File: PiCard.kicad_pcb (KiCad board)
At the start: 4 copper layers, 81 x 50 mm, 54 parts, among them J1 Usb Data Jumper, J2 USB_C_Receptacle_USB2.0_16P, J3 UART Activity Jumper, J4 Bus_M.2_Socket_M, J5 Ethernet, J6 Micro_SD_Card_Det2, J7 nRPIBOOT Jumper, J8 RS232, M2_3V3 TestPoint, U1 TPD4EUSB30, U3 TPD4EUSB30, U4 TPD4EUSB30, U5 MAX3232, U6 RT9742GGJ5, U7 TPS82130

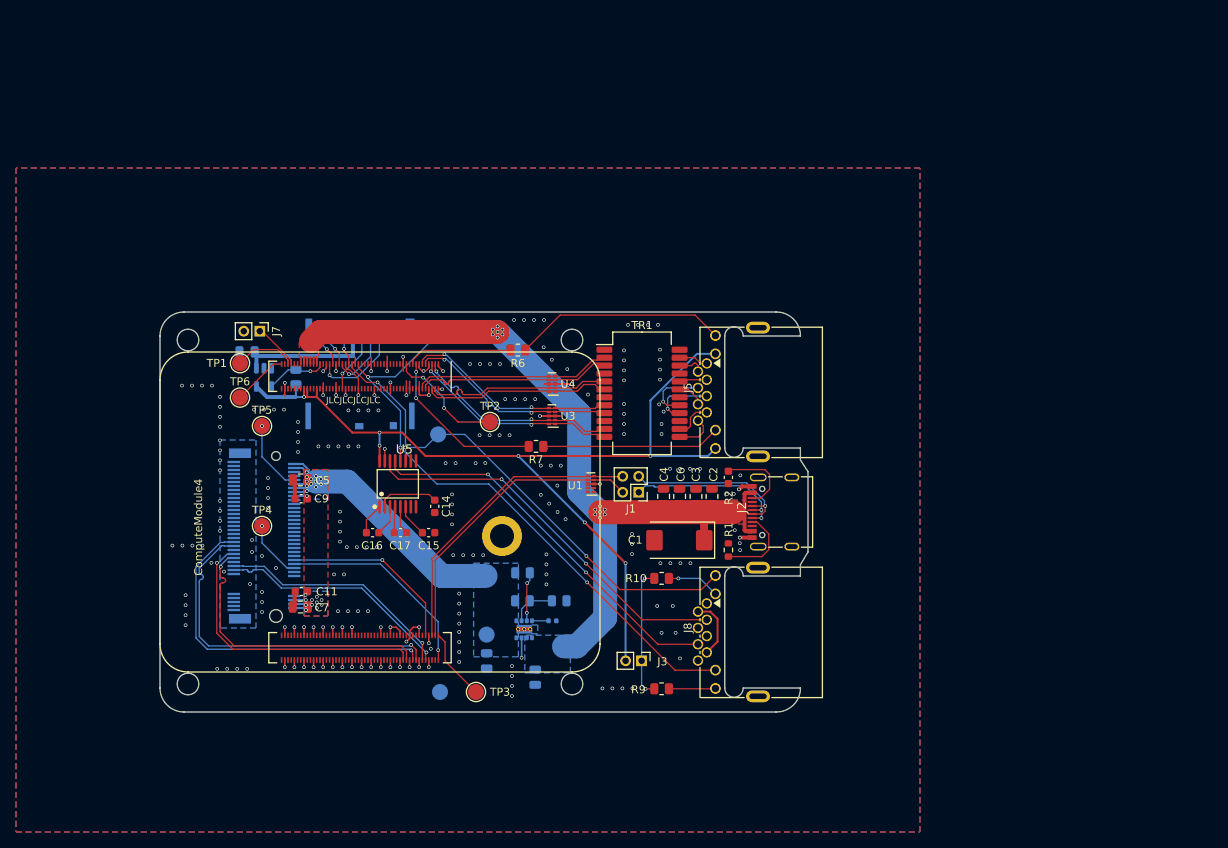
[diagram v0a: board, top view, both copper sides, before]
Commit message: update
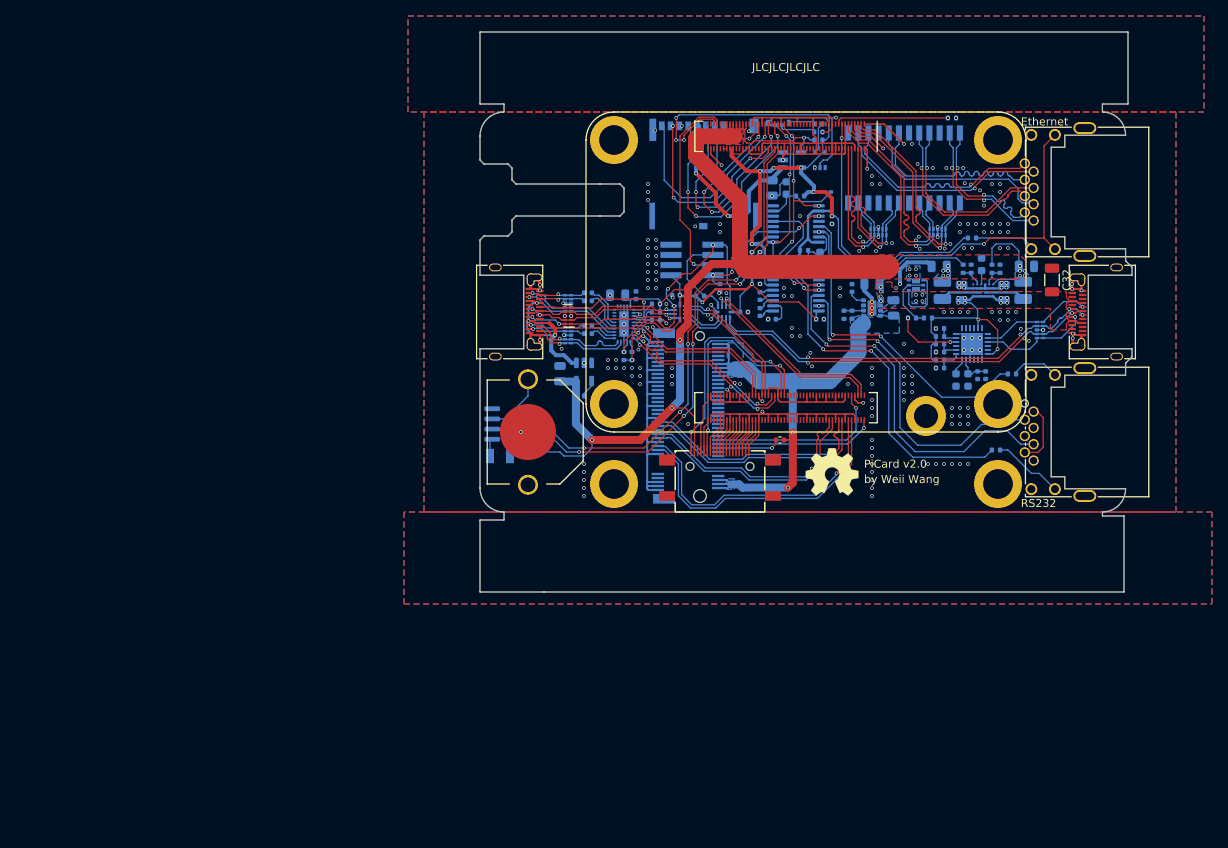
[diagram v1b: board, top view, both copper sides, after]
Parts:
- removed +5V1, GND1, GPIO14, GPIO15, M2_3V3, TP1, TP2, TP3, TP4, TP5, TP6: TestPoint, TestPoint:TestPoint_Pad_D2.0mm
- removed ComputeModule4: ComputeModule4-CM4, PiCard:Raspberry-Pi-4-Compute-Module
- removed J7: nRPIBOOT Jumper, Connector_PinHeader_2.00mm:PinHeader_1x02_P2.00mm_Vertical
- added BT1: RTC Battery, PiCard:BAT-SMD_MY-1220-03, F.Cu at (106.0, 90.0)
- added C13: 100n, Capacitor_SMD:C_0402_1005Metric, B.Cu at (163.2, 82.9)
- added C19: 22u, Capacitor_SMD:C_0805_2012Metric, B.Cu at (149.0, 71.5)
- added C20: 22u, Capacitor_SMD:C_0805_2012Metric, B.Cu at (151.7, 74.5)
- added C21: 430pF, Capacitor_SMD:C_0402_1005Metric, B.Cu at (146.5, 72.0)
- added C22: 100n, Capacitor_SMD:C_0402_1005Metric, B.Cu at (106.5, 92.5)
- added C23: 47u, Capacitor_SMD:C_0805_2012Metric, B.Cu at (110.0, 82.7)
- added C24: 47u, Capacitor_SMD:C_0805_2012Metric, B.Cu at (117.2, 72.9)
- added C25: 100n, Capacitor_SMD:C_0402_1005Metric, B.Cu at (119.5, 72.9)
- added C26: 100n, Capacitor_SMD:C_0402_1005Metric, B.Cu at (124.5, 72.9)
- added C27: 100n, Capacitor_SMD:C_0402_1005Metric, B.Cu at (113.5, 77.7)
- added C28: 100n, Capacitor_SMD:C_0402_1005Metric, B.Cu at (113.5, 76.7)
- added C29: 100n, Capacitor_SMD:C_0402_1005Metric, B.Cu at (133.0, 75.0)
- added C30: 100n, Capacitor_SMD:C_0402_1005Metric, B.Cu at (113.5, 72.6)
- added C31: 100n, Capacitor_SMD:C_0402_1005Metric, B.Cu at (113.5, 73.6)
- added C32: 2.2u, Capacitor_SMD:C_1206_3216Metric, F.Cu at (171.5, 71.0)
- added ComputeModule1: ComputeModule4-CM4, PiCard:Raspberry-Pi-4-Compute-Module, F.Cu at (116.8, 53.5)
- added D1: 1N5819WS, Diode_SMD:D_SOD-323, B.Cu at (140.0, 68.8)
- added D3: 1N5819WS, Diode_SMD:D_SOD-323, B.Cu at (142.8, 60.0)
- added D4: LED_Dual_AAKK, PiCard:LED-ARRAY-SMD_4P-L3.0-W1.5-L-FD, B.Cu at (137.3, 51.5)
- added H1: MountingHole, PiCard:MOUNTING-HOLE, F.Cu at (116.8, 96.5)
- added H2: MountingHole, PiCard:MOUNTING-HOLE, F.Cu at (164.8, 96.5)
- added L1: 1u, Inductor_SMD:L_1008_2520Metric, B.Cu at (167.9, 72.3)
- added L2: 1u, Inductor_SMD:L_1008_2520Metric, B.Cu at (157.8, 72.3)
- added Q1: DMP2065UFDB, PiCard:DFN200X200X60-8N, B.Cu at (154.5, 71.6)
- added R11: 680k 1%, Resistor_SMD:R_0402_1005Metric, B.Cu at (160.4, 69.6)
- added R12: 100k 1%, Resistor_SMD:R_0402_1005Metric, B.Cu at (161.4, 69.6)
- added R13: 5.1k, Resistor_SMD:R_0402_1005Metric, B.Cu at (157.5, 79.0)
- added R14: 1k, Resistor_SMD:R_0402_1005Metric, B.Cu at (157.5, 80.0)
- added R15: 150k 1%, Resistor_SMD:R_0402_1005Metric, B.Cu at (165.0, 69.6)
- added R17: 5.1k, Resistor_SMD:R_0402_1005Metric, B.Cu at (157.5, 81.0)
- added R18: 1k, Resistor_SMD:R_0402_1005Metric, B.Cu at (157.5, 82.0)
- added R19: 5.1k, Resistor_SMD:R_0402_1005Metric, B.Cu at (157.5, 78.1)
- added R20: 2.4k, Resistor_SMD:R_0402_1005Metric, B.Cu at (157.5, 77.1)
- added R22: 309k, Resistor_SMD:R_0402_1005Metric, B.Cu at (146.5, 75.3)
- added R23: 49.9k, Resistor_SMD:R_0402_1005Metric, B.Cu at (156.0, 75.7)
- added R24: 100k 1%, Resistor_SMD:R_0402_1005Metric, B.Cu at (145.5, 75.3)
- added R25: 1k, Resistor_SMD:R_0402_1005Metric, B.Cu at (154.0, 75.7)
- added R26: 5.1k, Resistor_SMD:R_0402_1005Metric, B.Cu at (135.0, 67.0)
- added R27: 5.1k, Resistor_SMD:R_0402_1005Metric, B.Cu at (134.0, 67.0)
- added R28: 12k, Resistor_SMD:R_0402_1005Metric, B.Cu at (112.5, 85.5)
- added R29: 909k, Resistor_SMD:R_0402_1005Metric, B.Cu at (122.0, 76.0)
- added R30: 12k, Resistor_SMD:R_0402_1005Metric, B.Cu at (127.5, 73.0)
- added R31: 200k, Resistor_SMD:R_0402_1005Metric, B.Cu at (119.0, 80.5)
- added R32: 200k, Resistor_SMD:R_0402_1005Metric, B.Cu at (122.0, 75.0)
- added R33: 499k, Resistor_SMD:R_0402_1005Metric, B.Cu at (122.0, 74.0)
- added R34: 12k, Resistor_SMD:R_0402_1005Metric, B.Cu at (118.0, 80.5)
- added R35: 12k, Resistor_SMD:R_0402_1005Metric, B.Cu at (130.0, 72.0)
- added R36: 1k, Resistor_SMD:R_0402_1005Metric, B.Cu at (142.3, 51.5)
- added SW1: SW_DIP_x04, PiCard:SW-SMD_8P-P1.27_EU-04KS, B.Cu at (126.5, 68.5)
- added SYM1: PiCard v2.0, PiCard:PICARD_NAMEPLATE, F.Cu at (144.0, 95.0)
- added U10: TPS2069C, Package_TO_SOT_SMD:SOT-23-5, B.Cu at (113.0, 82.5)
- added U11: TPD4EUSB30, Package_SON:USON-10_2.5x1.0mm_P0.5mm, B.Cu at (170.0, 77.2)
- added U12: TPD4EUSB30, Package_SON:USON-10_2.5x1.0mm_P0.5mm, F.Cu at (111.0, 75.5)
- added U13: TPD4EUSB30, Package_SON:USON-10_2.5x1.0mm_P0.5mm, B.Cu at (111.0, 77.9)
- added U14: TPD4EUSB30, Package_SON:USON-10_2.5x1.0mm_P0.5mm, B.Cu at (111.0, 73.9)
- added U15: TS3USB221, PiCard:RSE10, B.Cu at (130.5, 75.0)
- added U16: HD3SS3220, PiCard:RNH0030A, B.Cu at (118.0, 76.5)
- added U17: TS3USB221, PiCard:RSE10, B.Cu at (125.0, 75.0)
- added U18: 74LVC1G07, Package_TO_SOT_SMD:SOT-353_SC-70-5, B.Cu at (142.5, 56.0)
- added U2: SN74AHC123A, Package_SO:TSSOP-16_4.4x5mm_P0.65mm, B.Cu at (139.5, 64.0)
- added U8: TPS82130, PiCard:Texas_SIL0008D_MicroSiP-8-1EP_2.8x3mm_P0.65mm_EP1.1x1.9mm_ThermalVias, B.Cu at (149.0, 74.5)
- added U9: DS1307Z+, Package_SO:SOIC-8_3.9x4.9mm_P1.27mm, B.Cu at (104.0, 89.0)
- added Y1: 32.768kHz, Crystal:Crystal_SMD_3215-2Pin_3.2x1.5mm, B.Cu at (102.5, 93.0)
- C1: value 100uF -> 100n; footprint Capacitor_Tantalum_SMD:CP_EIA-7343-31_Kemet-D -> Capacitor_SMD:C_0402_1005Metric; moved to B.Cu
- C10: value 430pF -> 1u; footprint Capacitor_SMD:C_0402_1005Metric -> Capacitor_SMD:C_0603_1608Metric
- C11: value 100nF -> 1u; moved to B.Cu
- C12: value 22uF -> 100n; footprint Capacitor_SMD:C_0805_2012Metric -> Capacitor_SMD:C_0402_1005Metric
- C14, C15: value 100nF -> 22u; footprint Capacitor_SMD:C_0603_1608Metric -> Capacitor_SMD:C_0805_2012Metric; moved to B.Cu
- C16, C17: value 100nF -> 47u; footprint Capacitor_SMD:C_0603_1608Metric -> Capacitor_SMD:C_0805_2012Metric; moved to B.Cu
- C18: value 10uF -> 22n; footprint Capacitor_SMD:C_0805_2012Metric -> Capacitor_SMD:C_0603_1608Metric
- C2, C3, C4, C5, C7: value 10u -> 100n; footprint Capacitor_SMD:C_0805_2012Metric -> Capacitor_SMD:C_0402_1005Metric; moved to B.Cu
- C6: value 10u -> 1u; footprint Capacitor_SMD:C_0805_2012Metric -> Capacitor_SMD:C_0603_1608Metric; moved to B.Cu
- C8: value 22uF -> 1u; footprint Capacitor_SMD:C_0805_2012Metric -> Capacitor_SMD:C_0603_1608Metric
- C9: value 100nF -> 10u; footprint Capacitor_SMD:C_0603_1608Metric -> Capacitor_SMD:C_0805_2012Metric; moved to B.Cu
- J1: value Usb Data Jumper -> RS232; footprint Connector_PinHeader_2.00mm:PinHeader_2x02_P2.00mm_Vertical -> PiCard:RJ45-TH_RJ45-005-202-11
- J2: value USB_C_Receptacle_USB2.0_16P -> Ethernet; footprint PiCard:USB-C-SMD_TYPEC-304J-BCP16 -> PiCard:RJ45-TH_RJ45-005-202-11
- J3: value UART Activity Jumper -> Micro_SD_Card_Det2; footprint Connector_PinHeader_2.00mm:PinHeader_1x02_P2.00mm_Vertical -> PiCard:TF-SMD_503398-1892; moved to B.Cu
- J5: value Ethernet -> USB_C_Receptacle; footprint PiCard:RJ45-TH_MJ88B-B011-RVL11-P -> PiCard:USB-C-SMD_TYPE-C-31-M-27
- J6: value Micro_SD_Card_Det2 -> USB_C_Receptacle; footprint PiCard:TF-SMD_503398-1892 -> PiCard:USB-C-SMD_TYPE-C-31-M-27; moved to F.Cu
- J8: value RS232 -> HDMI_C_1.4; footprint PiCard:RJ45-TH_MJ88B-B011-RVL11-P -> PiCard:HDMI-SMD_19P-P0.40-H-F_HDMI-519S
- R1: value 5.1K -> 470; footprint Resistor_SMD:R_0603_1608Metric -> Resistor_SMD:R_0402_1005Metric; moved to B.Cu
- R10: value 470R -> 787k; footprint Resistor_SMD:R_0805_2012Metric -> Resistor_SMD:R_0402_1005Metric; moved to B.Cu
- R2: value 5.1K -> 470; footprint Capacitor_SMD:C_0603_1608Metric -> Resistor_SMD:R_0402_1005Metric; moved to B.Cu
- R3: value 100k -> 1k; footprint Resistor_SMD:R_0805_2012Metric -> Resistor_SMD:R_0402_1005Metric
- R4: value 309k -> 100k 1%; footprint Resistor_SMD:R_0805_2012Metric -> Resistor_SMD:R_0402_1005Metric
- R5: value 100k -> 100k 1%; footprint Resistor_SMD:R_0805_2012Metric -> Resistor_SMD:R_0402_1005Metric
- R6, R7: value 470R -> 470; footprint Resistor_SMD:R_0805_2012Metric -> Resistor_SMD:R_0402_1005Metric; moved to B.Cu
- R8: value 12K 1% -> 12k; footprint Resistor_SMD:R_0805_2012Metric -> Resistor_SMD:R_0402_1005Metric
- R9: value 470R -> 12k; footprint Resistor_SMD:R_0805_2012Metric -> Resistor_SMD:R_0402_1005Metric
- TR1: value 30F-51NL -> H2456G; footprint Transformer_SMD:Transformer_Ethernet_YDS_30F-51NL_SO-24_7.1x15.1mm -> PiCard:XFMR-SMD-24_L16.6-W9.0-LS9.6-BL; moved to B.Cu
- U1: value TPD4EUSB30 -> MAX3232; footprint Package_SON:USON-10_2.5x1.0mm_P0.5mm -> Package_SO:TSSOP-16_4.4x5mm_P0.65mm; moved to B.Cu
- U3, U4: moved to B.Cu
- U5: value MAX3232 -> RT9742GGJ5; footprint PiCard:TSSOP-16_L5.0-W4.4-P0.65-LS6.4-BL -> Package_TO_SOT_SMD:TSOT-23-5; moved to B.Cu
- U6: value RT9742GGJ5 -> TPS62180; footprint Package_TO_SOT_SMD:TSOT-23-5 -> PiCard:YZF0024AMAM
- U7: value TPS82130 -> CYPD3177-24LQ; footprint PiCard:Texas_SIL0008D_MicroSiP-8-1EP_2.8x3mm_P0.65mm_EP1.1x1.9mm_ThermalVias -> Package_DFN_QFN:QFN-24-1EP_4x4mm_P0.5mm_EP2.75x2.75mm
- moved C18 92.5 mm to (162.7, 69.0), turned to 90 degrees
- moved J6 92.1 mm to (176.8, 75.0), turned to 90 degrees
- moved U6 90.6 mm to (162.9, 72.3), turned to 90 degrees
- moved C16 88.2 mm to (168.3, 69.3)
- moved C11 87.4 mm to (161.0, 83.5), turned to 90 degrees
- moved C7 82.2 mm to (144.0, 63.5), turned to 90 degrees
- moved C14 76.0 mm to (165.5, 72.5), turned to 90 degrees
- moved C17 75.1 mm to (157.4, 69.3), turned to 180 degrees
- moved C15 73.1 mm to (160.2, 72.5), turned to 90 degrees
- moved R8 71.7 mm to (142.3, 53.5), turned to 0 degrees
- moved C12 71.0 mm to (162.2, 82.9), turned to 90 degrees
- moved C9 70.5 mm to (136.5, 59.5), turned to -90 degrees
- moved C8 68.7 mm to (138.3, 59.5), turned to 90 degrees
- moved U7 66.4 mm to (161.5, 79.0), turned to 0 degrees
- moved R3 66.4 mm to (142.3, 52.5), turned to 180 degrees
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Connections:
- C1 pad 1: +5V -> GND
- C1 pad 2: GND -> +3.3V
- C10 pad 2: Net-(U7-SS/TR) -> Net-(U7-VCCD)
- C11 pad 1: /Module B/M2_3V3 -> GND
- C11 pad 2: GND -> Net-(U7-VDDD)
- C12 pad 1: /Module B/M2_3V3 -> GND
- C12 pad 2: GND -> Net-(U7-VDDD)
- C14 pad 1: Net-(U5-VS+) -> VBUS
- C15 pad 1: Net-(U5-VS-) -> VBUS
- C16 pad 1: Net-(U5-C1+) -> +5V
- C16 pad 2: Net-(U5-C1-) -> GND
- C17 pad 1: Net-(U5-C2+) -> +5V
- C17 pad 2: Net-(U5-C2-) -> GND
- C18 pad 1: /Module A/SD_PWR -> Net-(U6-SS)
- C2 pad 1: +5V -> Net-(U1-C1+)
- C2 pad 2: GND -> Net-(U1-C1-)
- C3 pad 1: +5V -> Net-(U1-C2+)
- C3 pad 2: GND -> Net-(U1-C2-)
- C4 pad 1: +5V -> Net-(U1-VS+)
- C5 pad 1: GND -> Net-(U1-VS-)
- C5 pad 2: /Module B/M2_3V3 -> GND
- C6 pad 1: +5V -> Net-(D1-A)
- C7 pad 2: /Module B/M2_3V3 -> +3.3V
- C8 pad 1: +5V -> Net-(D3-A)
- C9 pad 1: /Module B/M2_3V3 -> /Module A/SD_PWR
- J1 pad 2: /Module B/USB2_N -> Net-(J1-Pad2)
- J1 pad 3: /Module B/TYPEC_D_P -> /Module A/RS232_TXD
- J1 pad 4: /Module B/USB2_P -> GND
- J3 pad 1: Net-(J3-Pin_1) -> /Module A/SD_DAT2
- J3 pad 2: +3.3V -> /Module A/SD_DAT3
- J4 pad 10: /Module B/M2_LED -> unconnected-(J4-DAS/~{DSS}/~{LED1}-Pad10)
- J4 pad 12: /Module B/M2_3V3 -> M2_3.3V
- J4 pad 14: /Module B/M2_3V3 -> M2_3.3V
- J4 pad 16: /Module B/M2_3V3 -> M2_3.3V
- J4 pad 18: /Module B/M2_3V3 -> M2_3.3V
- J4 pad 2: /Module B/M2_3V3 -> M2_3.3V
- J4 pad 4: /Module B/M2_3V3 -> M2_3.3V
- J4 pad 54: /Module B/PEWAKE -> Net-(J4-~{PEWAKE})
- J4 pad 70: /Module B/M2_3V3 -> M2_3.3V
- J4 pad 72: /Module B/M2_3V3 -> M2_3.3V
- J4 pad 74: /Module B/M2_3V3 -> M2_3.3V
- J8 pad 1: unconnected-(J8-Pad1) -> GND
- J8 pad 10: Net-(J8-Pad10) -> GND
- J8 pad 11: /Module A/GPIO14_UART_TX -> /Module B/HDMI0_CLK_P
- J8 pad 12: Net-(J8-Pad12) -> /Module B/HDMI0_CLK_N
- J8 pad 2: Net-(J8-Pad2) -> /Module B/HDMI0_TX2_P
- J8 pad 3: /Module A/RS232_TXD -> /Module B/HDMI0_TX2_N
- J8 pad 5: GND -> /Module B/HDMI0_TX1_P
- J8 pad 6: /Module A/RS232_RXD -> /Module B/HDMI0_TX1_N
- J8 pad 7: Net-(J8-Pad2) -> GND
- J8 pad 8: unconnected-(J8-Pad8) -> /Module B/HDMI0_TX0_P
- J8 pad 9: /Module A/GPIO15_UART_RX -> /Module B/HDMI0_TX0_N
- R1 pad 1: Net-(J2-CC1) -> Net-(J1-Pad12)
- R1 pad 2: GND -> /Module A/UART_TX_ACT
- R10 pad 1: Net-(J8-Pad12) -> +5V
- R10 pad 2: Net-(J3-Pin_1) -> Net-(U6-FB)
- R2 pad 1: GND -> /Module A/UART_RX_ACT
- R2 pad 2: Net-(J2-CC2) -> Net-(J1-Pad10)
- R3 pad 1: /Module B/M2_3V3 -> /Module A/GREEN_LED_K
- R3 pad 2: Net-(U7-PG) -> Net-(D4-K2)
- R4 pad 1: /Module B/M2_3V3 -> +3.3V
- R4 pad 2: Net-(U7-FB) -> Net-(D1-A)
- R5 pad 1: GND -> +3.3V
- R5 pad 2: Net-(U7-FB) -> Net-(D3-A)
- R6 pad 1: Net-(J5-Pad11) -> Net-(J2-Pad11)
- R7 pad 1: Net-(J5-Pad9) -> Net-(J2-Pad9)
- R8 pad 1: +3.3V -> /Module A/SD_PWR_ON
- R8 pad 2: /Module A/SD_PWR_ON -> +3.3V
- R9 pad 1: Net-(J3-Pin_1) -> Net-(J4-~{PEWAKE})
- R9 pad 2: Net-(J8-Pad10) -> M2_3.3V
- TR1 pad 11: /Module A/TRD3_P -> /Module A/DD_N
- TR1 pad 12: /Module A/TRD3_N -> /Module A/DD_P
- TR1 pad 13: /Module A/DD_N -> /Module A/TRD3_P
- TR1 pad 14: /Module A/DD_P -> /Module A/TRD3_N
- TR1 pad 16: /Module A/DC_N -> /Module A/TRD2_P
- TR1 pad 17: /Module A/DC_P -> /Module A/TRD2_N
- TR1 pad 19: /Module A/DB_N -> /Module A/TRD1_P
- TR1 pad 2: /Module A/TRD0_P -> /Module A/DA_N
- TR1 pad 20: /Module A/DB_P -> /Module A/TRD1_N
- TR1 pad 22: /Module A/DA_N -> /Module A/TRD0_P
- TR1 pad 23: /Module A/DA_P -> /Module A/TRD0_N
- TR1 pad 3: /Module A/TRD0_N -> /Module A/DA_P
- TR1 pad 5: /Module A/TRD1_P -> /Module A/DB_N
- TR1 pad 6: /Module A/TRD1_N -> /Module A/DB_P
- TR1 pad 8: /Module A/TRD2_P -> /Module A/DC_N
- TR1 pad 9: /Module A/TRD2_N -> /Module A/DC_P
- U1 pad 1: unconnected-(U1-D1+-Pad1) -> Net-(U1-C1+)
- U1 pad 2: unconnected-(U1-D1--Pad2) -> Net-(U1-VS+)
- U1 pad 3: GND -> Net-(U1-C1-)
- U1 pad 4: /Module B/USB2_N -> Net-(U1-C2+)
- U1 pad 5: /Module B/USB2_P -> Net-(U1-C2-)
- U1 pad 6: /Module B/USB2_P -> Net-(U1-VS-)
- U1 pad 7: /Module B/USB2_N -> unconnected-(U1-T2OUT-Pad7)
- U1 pad 8: GND -> unconnected-(U1-R2IN-Pad8)
- U3 pad 1: /Module A/TRD3_N -> /Module A/TRD3_P
- U3 pad 10: /Module A/TRD3_N -> /Module A/TRD3_P
- U3 pad 2: /Module A/TRD3_P -> /Module A/TRD3_N
- U3 pad 4: /Module A/TRD2_N -> /Module A/TRD2_P
- U3 pad 5: /Module A/TRD2_P -> /Module A/TRD2_N
- U3 pad 6: /Module A/TRD2_P -> /Module A/TRD2_N
- U3 pad 7: /Module A/TRD2_N -> /Module A/TRD2_P
- U3 pad 9: /Module A/TRD3_P -> /Module A/TRD3_N
- U4 pad 1: /Module A/TRD1_N -> /Module A/TRD0_N
- U4 pad 10: /Module A/TRD1_N -> /Module A/TRD0_N
- U4 pad 2: /Module A/TRD1_P -> /Module A/TRD0_P
- U4 pad 4: /Module A/TRD0_N -> /Module A/TRD1_N
- U4 pad 5: /Module A/TRD0_P -> /Module A/TRD1_P
- U4 pad 6: /Module A/TRD0_P -> /Module A/TRD1_P
- U4 pad 7: /Module A/TRD0_N -> /Module A/TRD1_N
- U4 pad 9: /Module A/TRD1_P -> /Module A/TRD0_P
- U5 pad 1: Net-(U5-C1+) -> /Module A/SD_PWR
- U5 pad 2: Net-(U5-VS+) -> GND
- U5 pad 3: Net-(U5-C1-) -> unconnected-(U5-~{FLG}-Pad3)
- U5 pad 4: Net-(U5-C2+) -> /Module A/SD_PWR_ON
- U5 pad 5: Net-(U5-C2-) -> +3.3V
- U7 pad 1: +5V -> Net-(U7-VBUS_MIN)
- U7 pad 2: +5V -> Net-(U7-VBUS_MAX)
- U7 pad 3: GND -> unconnected-(U7-VBUS_FET_EN-Pad3)
- U7 pad 4: /Module B/M2_3V3 -> /Power/SAFE_PWR_EN
- U7 pad 5: /Module B/M2_3V3 -> Net-(U7-ISNK_COARSE)
- U7 pad 6: Net-(U7-FB) -> GND
- U7 pad 7: Net-(U7-PG) -> unconnected-(U7-~{HPI_INT}-Pad7)
- U7 pad 8: Net-(U7-SS/TR) -> unconnected-(U7-GPIO_1-Pad8)
- U7 pad 9: GND -> unconnected-(U7-FAULT-Pad9)
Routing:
- net GND: track 83.2 -> 255.0 mm, vias 229 -> 216
- net RTC_SCL: track 0.00 -> 63.9 mm, vias 0 -> 5
- net RTC_SDA: track 0.00 -> 63.2 mm, vias 0 -> 5
- net M2_3.3V: track 0.00 -> 60.4 mm, vias 0 -> 2
- net /Module A/UART_RX_ACT: track 0.00 -> 54.1 mm, vias 0 -> 2
- net /USB/RIGHT_USB2_P: track 0.00 -> 50.5 mm, vias 0 -> 3
- net /USB/RIGHT_USB2_N: track 0.00 -> 50.4 mm, vias 0 -> 4
- net /Module A/GPIO15_UART_RX: track 76.6 -> 28.3 mm, vias 3 -> 6
- net +3.3V: track 118.4 -> 164.5 mm, vias 7 -> 13
- net VBUS: track 0.00 -> 44.5 mm, vias 0 -> 18
- net /USB/USB3_VBUS: track 0.00 -> 43.6 mm, vias 0 -> 4
- net /Module B/M2_3V3: track 42.2 -> 0.00 mm, vias 24 -> 0
- net /Module A/UART_TX_ACT: track 0.00 -> 41.0 mm, vias 0 -> 2
- net /Module B/USB2_P: track 37.7 -> 0.00 mm
- net /Module A/GPIO14_UART_TX: track 63.9 -> 26.2 mm, vias 3 -> 5
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- added copper zone on B.Cu, net M2_3.3V
- added copper zone on B.Cu, net VBUS
- added copper zone on F.Cu, net VBUS
- removed copper zone on B.Cu, net /Module B/M2_3V3
- removed copper zone on F.Cu, net /Module B/M2_3V3
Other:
- board size 81 x 50 mm -> 81.5 x 70 mm
- board text added: "Ethernet"
- board text added: "RS232"
